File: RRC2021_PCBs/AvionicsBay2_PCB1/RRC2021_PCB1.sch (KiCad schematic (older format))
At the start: 14 parts, among them U1 ADXL357z, U2 MS5611

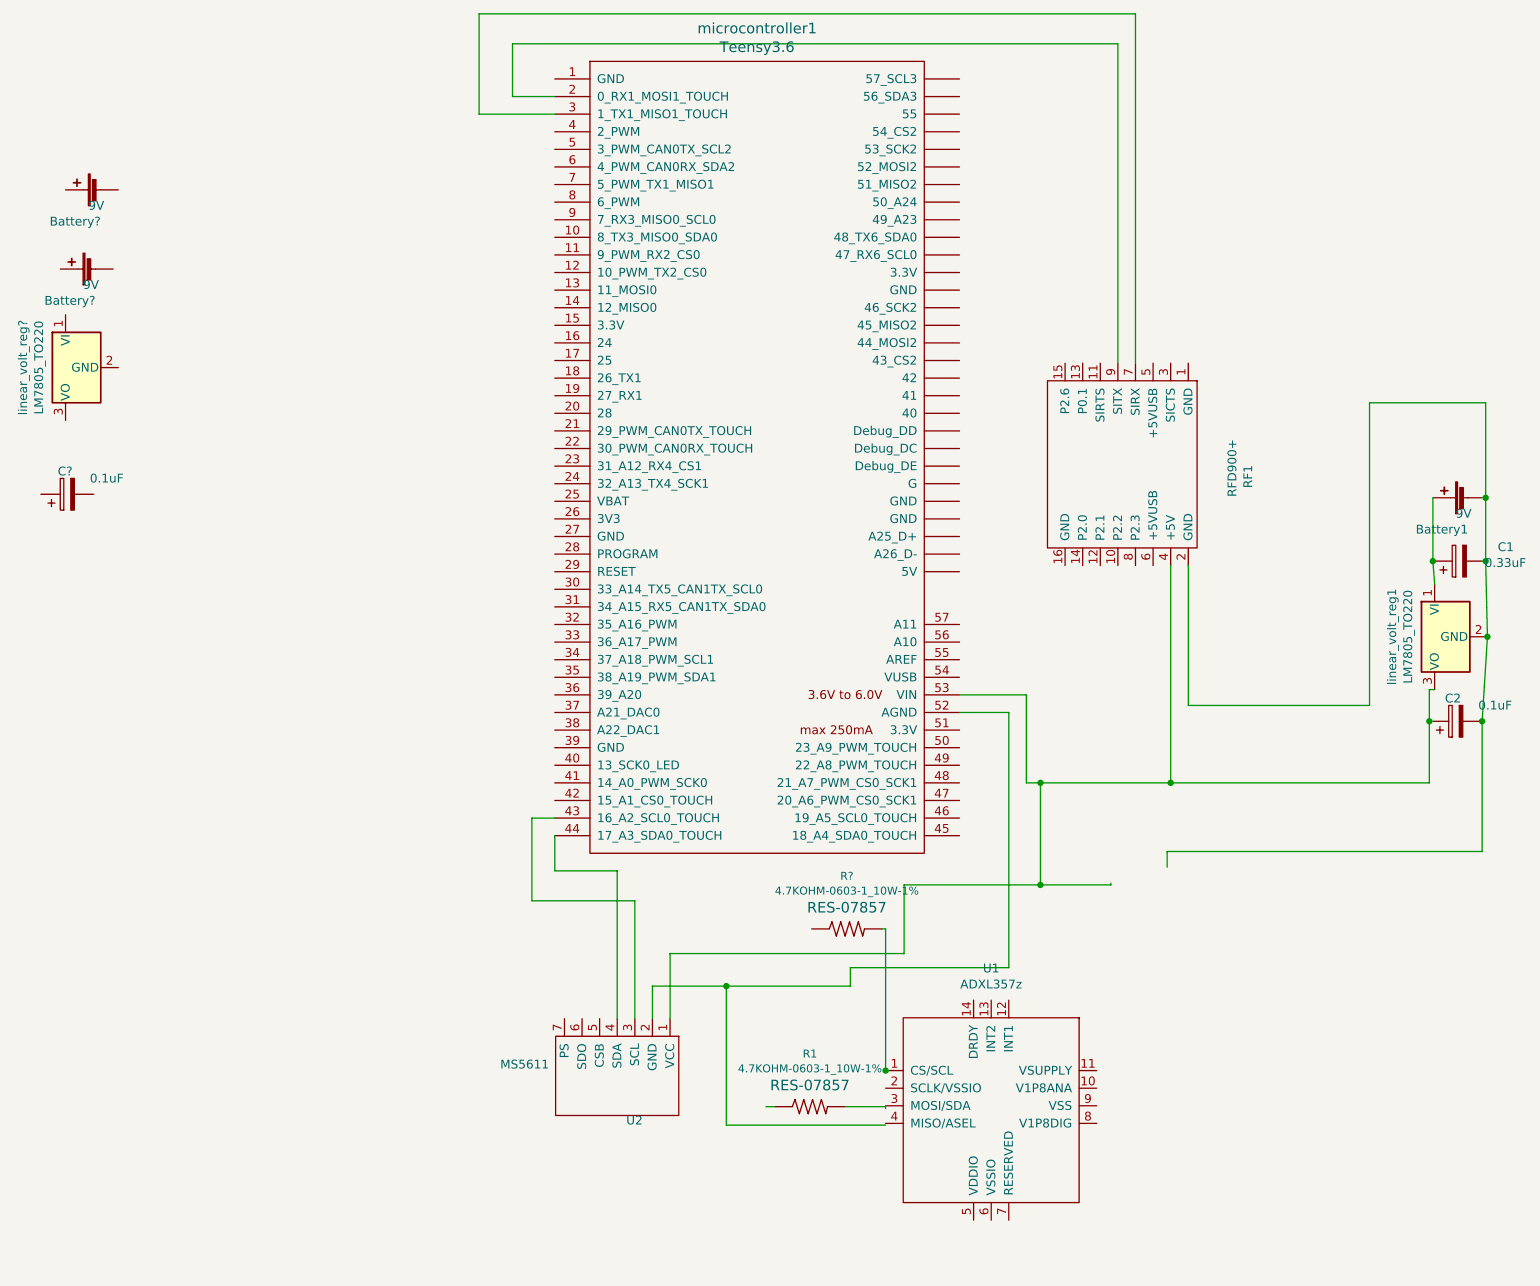
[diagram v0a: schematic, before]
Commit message: update
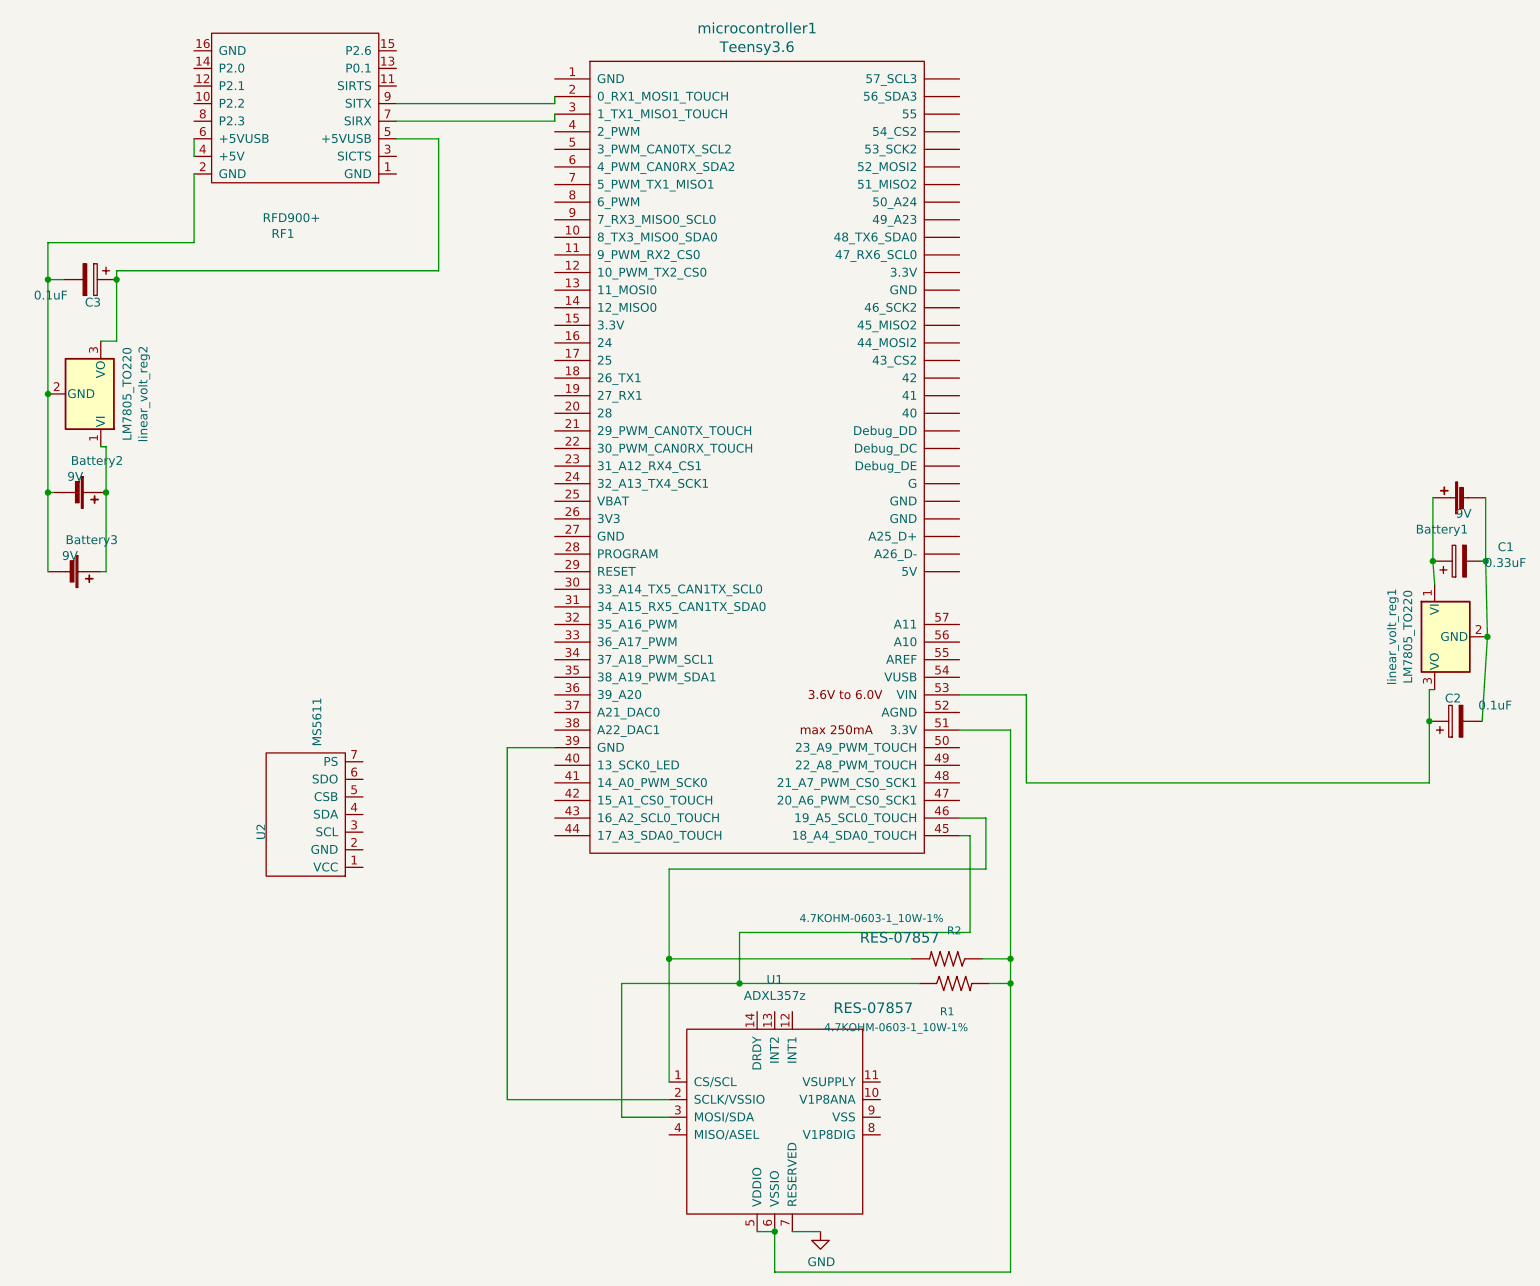
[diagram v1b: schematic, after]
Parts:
- gave numbers to parts that had none: 5
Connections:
- net labels added: GND
- wire segments 59 -> 61
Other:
- moved on the sheet: Battery2, Battery3, C3, R1, R2, RF1, U1, U2, linear_volt_reg2
